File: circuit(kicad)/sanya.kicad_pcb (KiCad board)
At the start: 2 copper layers, 34.4 x 27.8 mm, 10 parts, among them J1 Oled, J2 Micro_SD_Card, SW1 Up, SW2 Down, SW3 Set, SW4 SW_DPDT_x2, U1 ATmega328P-A

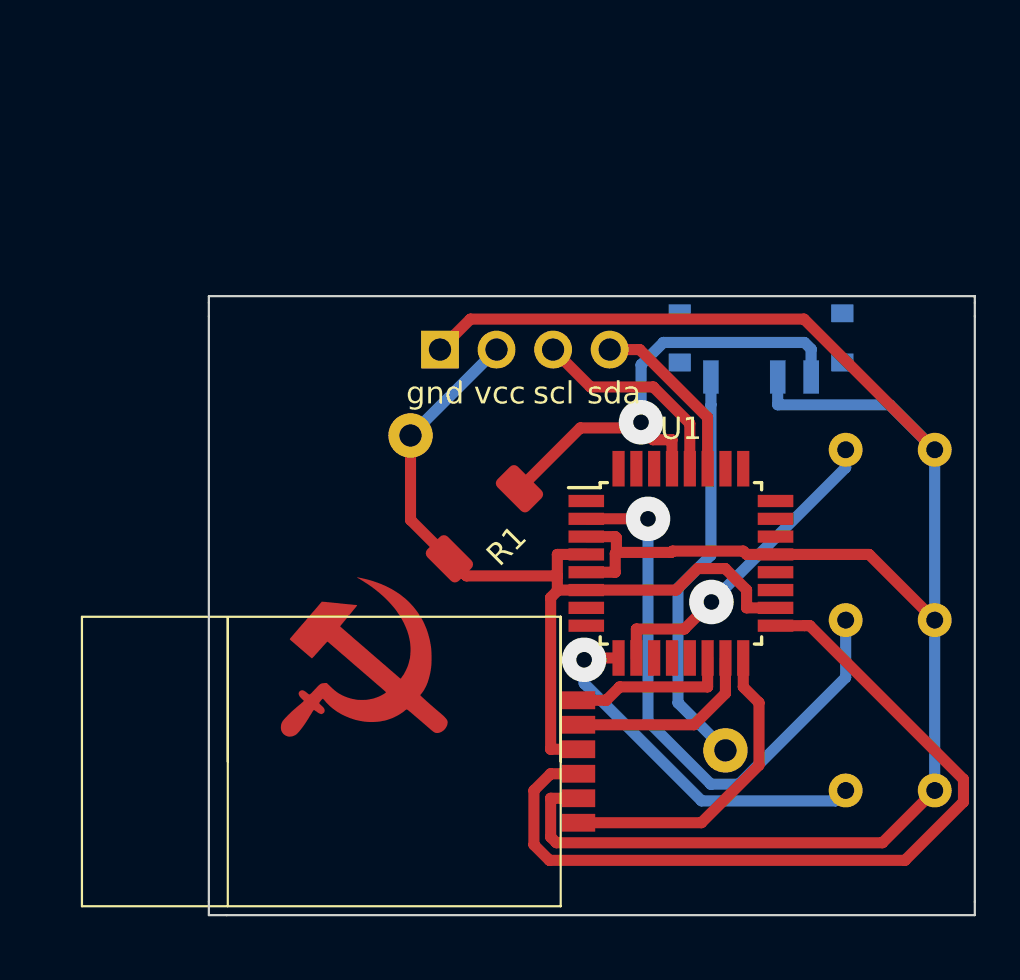
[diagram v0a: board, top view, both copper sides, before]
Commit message: подвигал дорожки, добавил лого :)
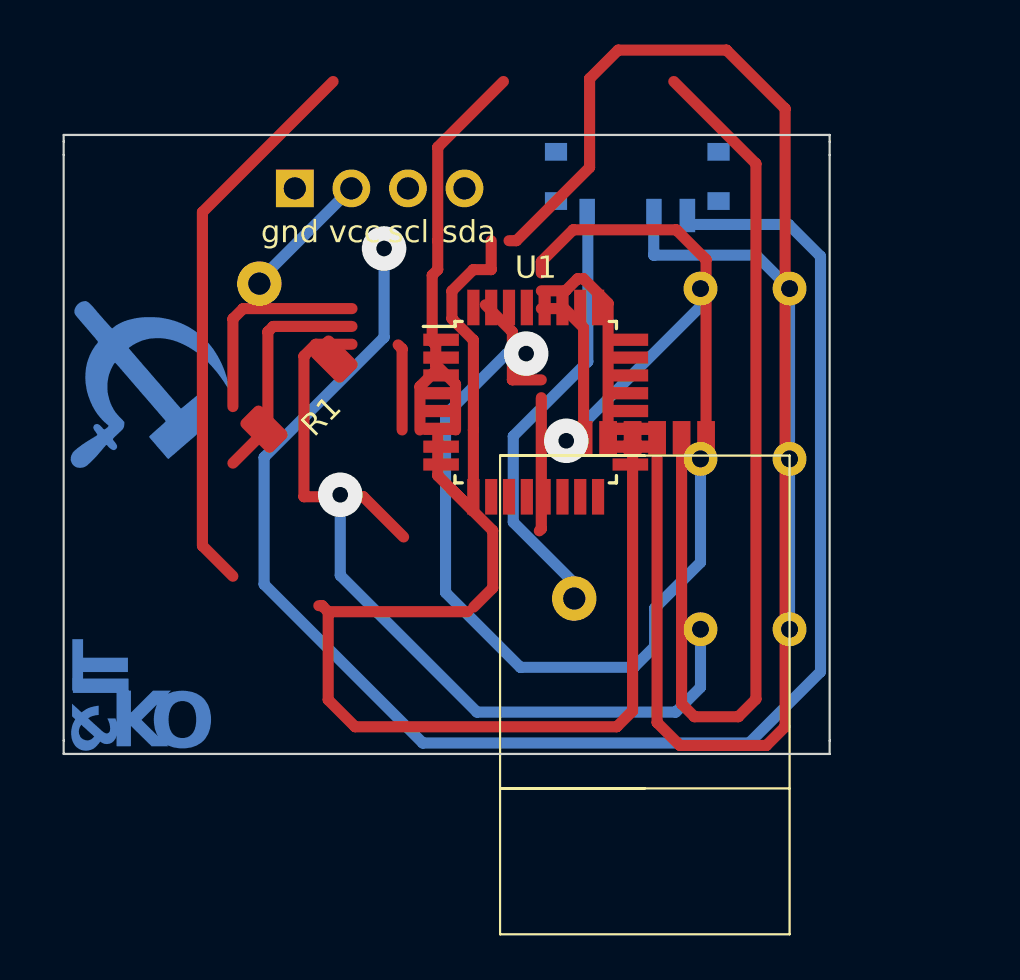
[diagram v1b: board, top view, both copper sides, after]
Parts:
- G***: moved to B.Cu
- moved G*** 15.5 mm to (141.2, 58.6), turned to 90 degrees
- moved J2 14.3 mm to (163.4, 61.8), turned to 0 degrees
- moved R1 10.2 mm to (147.8, 59.0)
- moved SW3 9.74 mm to (167.9, 61.9)
- moved J1 9.74 mm to (150.2, 49.8)
- moved SW1 9.74 mm to (167.9, 54.3)
- moved SW2 9.74 mm to (167.9, 69.6)
- moved U1 9.74 mm to (158.5, 59.4)
- moved BT1 9.62 mm to (148.9, 56.9)
- moved SW4 9.14 mm to (163.0, 49.5)
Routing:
- net /RST: track 21.8 -> 86.0 mm
- net VCC: track 39.7 -> 87.4 mm
- net /SCK: track 37.7 -> 66.4 mm
- net Earth: track 90.8 -> 115.2 mm
- net /PD5: track 16.8 -> 31.4 mm
- net /SCL: track 9.55 -> 0.00 mm
- net /SDA: track 7.96 -> 0.00 mm
- net /PD4: track 26.5 -> 33.2 mm
- net unconnected-(U1-XTAL2/PB7-Pad8): track 0.00 -> 3.89 mm
- net /MISO: track 14.3 -> 17.1 mm
- net Net-(BT1--): track 18.3 -> 19.4 mm
- net /MOSI: track 8.78 -> 9.72 mm
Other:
- board text added: "&"
- board text added: "I"
- board text added: "K"
- board text added: "O"
- board text added: "T"
